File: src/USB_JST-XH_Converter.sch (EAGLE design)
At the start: 47 parts, among them SW1 SS-12D00G3, U1 TCKE805NAWSON10B_TOS-REC, U2 TLP293

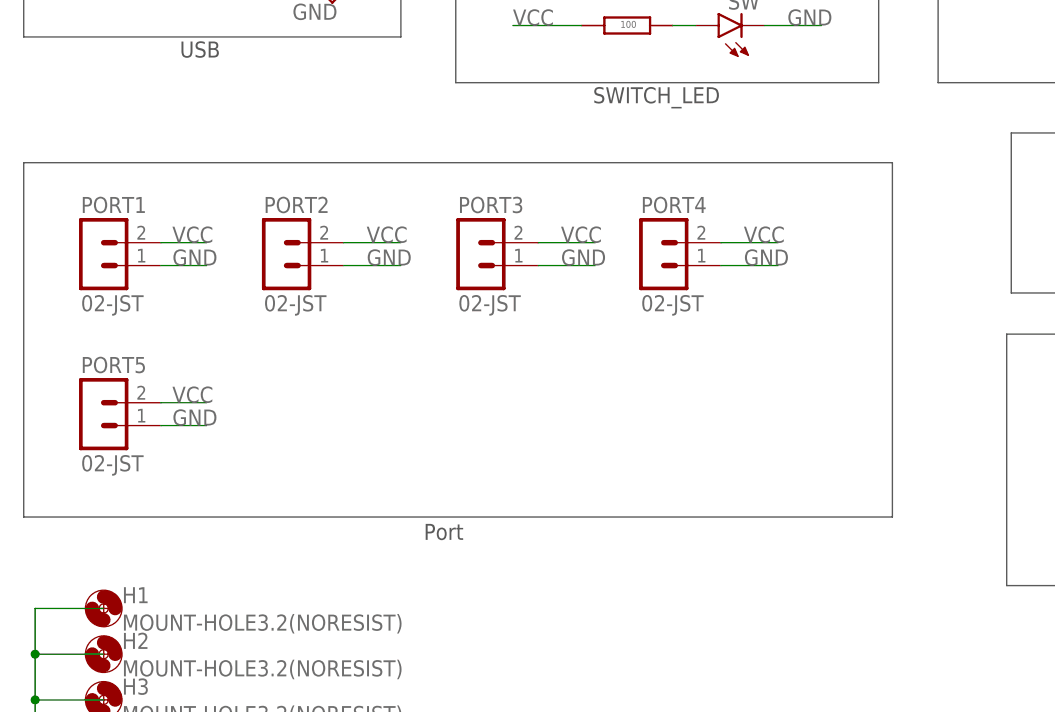
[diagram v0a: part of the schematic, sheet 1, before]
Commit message: 配線完了
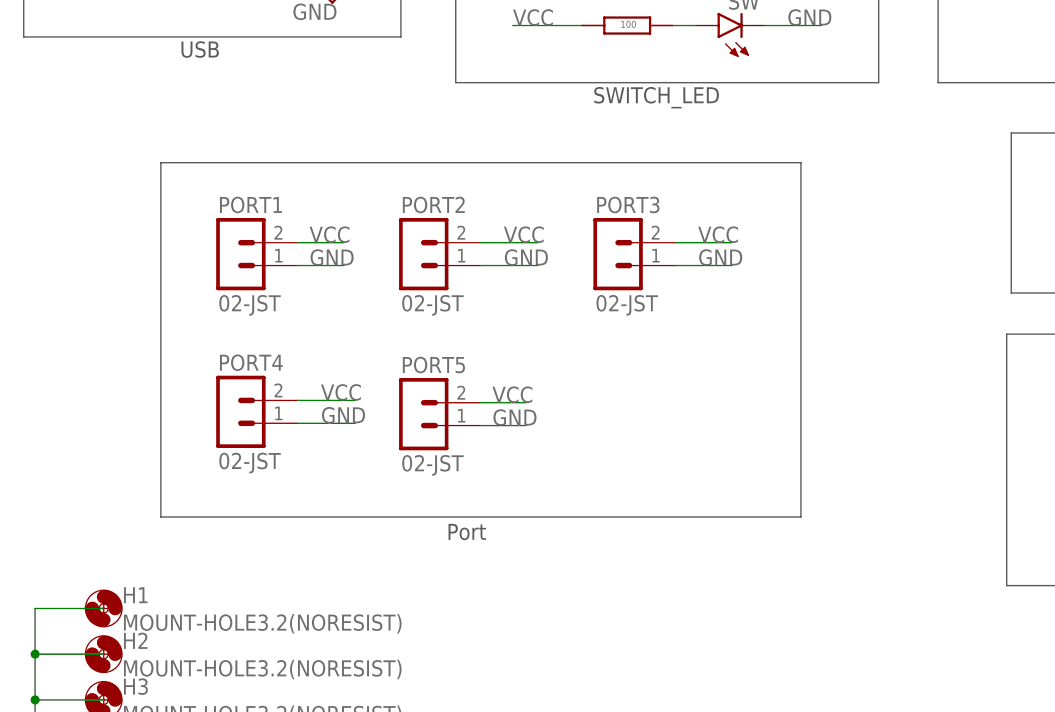
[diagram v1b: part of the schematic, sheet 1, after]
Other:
- moved on the sheet: PORT1, PORT2, PORT3, PORT4, PORT5
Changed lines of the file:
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@@
 <sheet>
 <plain>
-<wire x1="8.89" y1="74.93" x2="8.89" y2="35.56" width="0.1524" layer="97"/>
-<wire x1="8.89" y1="35.56" x2="105.41" y2="35.56" width="0.1524" layer="97"/>
-<wire x1="105.41" y1="35.56" x2="105.41" y2="74.93" width="0.1524" layer="97"/>
-<wire x1="105.41" y1="74.93" x2="8.89" y2="74.93" width="0.1524" layer="97"/>
+<wire x1="24.13" y1="74.93" x2="24.13" y2="35.56" width="0.1524" layer="97"/>
+<wire x1="24.13" y1="35.56" x2="95.25" y2="35.56" width="0.1524" layer="97"/>
+<wire x1="95.25" y1="35.56" x2="95.25" y2="74.93" width="0.1524" layer="97"/>
+<wire x1="95.25" y1="74.93" x2="24.13" y2="74.93" width="0.1524" layer="97"/>
 <wire x1="118.11" y1="55.88" x2="118.11" y2="27.94" width="0.1524" layer="97"/>
 <wire x1="118.11" y1="27.94" x2="170.18" y2="27.94" width="0.1524" layer="97"/>
@@
 <wire x1="170.18" y1="55.88" x2="118.11" y2="55.88" width="0.1524" layer="97"/>
 <text x="139.7" y="25.4" size="1.778" layer="97">Switch</text>
-<text x="53.34" y="33.02" size="1.778" layer="97">Port</text>
+<text x="55.88" y="33.02" size="1.778" layer="97">Port</text>
 <text x="30.734" y="86.614" size="1.778" layer="97" rot="MR0">USB</text>
 <wire x1="56.896" y1="97.79" x2="56.896" y2="83.82" width="0.1524" layer="97"/>
@@
 <attribute name="SHEET" x="154.305" y="5.08" size="2.54" layer="94"/>
 </instance>
-<instance part="PORT1" gate="G$1" x="16.51" y="66.04" smashed="yes">
-<attribute name="VALUE" x="15.24" y="58.42" size="1.778" layer="96"/>
-<attribute name="NAME" x="15.24" y="69.342" size="1.778" layer="95"/>
-</instance>
-<instance part="PORT2" gate="G$1" x="36.83" y="66.04" smashed="yes">
-<attribute name="VALUE" x="35.56" y="58.42" size="1.778" layer="96"/>
-<attribute name="NAME" x="35.56" y="69.342" size="1.778" layer="95"/>
-</instance>
-<instance part="PORT3" gate="G$1" x="58.42" y="66.04" smashed="yes">
-<attribute name="VALUE" x="57.15" y="58.42" size="1.778" layer="96"/>
-<attribute name="NAME" x="57.15" y="69.342" size="1.778" layer="95"/>
-</instance>
-<instance part="PORT4" gate="G$1" x="78.74" y="66.04" smashed="yes">
-<attribute name="VALUE" x="77.47" y="58.42" size="1.778" layer="96"/>
-<attribute name="NAME" x="77.47" y="69.342" size="1.778" layer="95"/>
-</instance>
-<instance part="PORT5" gate="G$1" x="16.51" y="48.26" smashed="yes">
-<attribute name="VALUE" x="15.24" y="40.64" size="1.778" layer="96"/>
-<attribute name="NAME" x="15.24" y="51.562" size="1.778" layer="95"/>
+<instance part="PORT1" gate="G$1" x="31.75" y="66.04" smashed="yes">
+<attribute name="VALUE" x="30.48" y="58.42" size="1.778" layer="96"/>
+<attribute name="NAME" x="30.48" y="69.342" size="1.778" layer="95"/>
+</instance>
+<instance part="PORT2" gate="G$1" x="52.07" y="66.04" smashed="yes">
+<attribute name="VALUE" x="50.8" y="58.42" size="1.778" layer="96"/>
+<attribute name="NAME" x="50.8" y="69.342" size="1.778" layer="95"/>
+</instance>
+<instance part="PORT3" gate="G$1" x="73.66" y="66.04" smashed="yes">
+<attribute name="VALUE" x="72.39" y="58.42" size="1.778" layer="96"/>
+<attribute name="NAME" x="72.39" y="69.342" size="1.778" layer="95"/>
+</instance>
+<instance part="PORT4" gate="G$1" x="31.75" y="48.514" smashed="yes">
+<attribute name="VALUE" x="30.48" y="40.894" size="1.778" layer="96"/>
+<attribute name="NAME" x="30.48" y="51.816" size="1.778" layer="95"/>
+</instance>
+<instance part="PORT5" gate="G$1" x="52.07" y="48.26" smashed="yes">
+<attribute name="VALUE" x="50.8" y="40.64" size="1.778" layer="96"/>
+<attribute name="NAME" x="50.8" y="51.562" size="1.778" layer="95"/>
 </instance>
 <instance part="SW1" gate="G$1" x="143.51" y="43.18" smashed="yes" rot="R270">
@@
 <segment>
 <pinref part="PORT1" gate="G$1" pin="2"/>
-<wire x1="24.13" y1="66.04" x2="29.21" y2="66.04" width="0.1524" layer="91"/>
-<label x="25.4" y="66.04" size="1.778" layer="95"/>
+<wire x1="39.37" y1="66.04" x2="44.45" y2="66.04" width="0.1524" layer="91"/>
+<label x="40.64" y="66.04" size="1.778" layer="95"/>
 </segment>
 <segment>
 <pinref part="PORT2" gate="G$1" pin="2"/>
-<wire x1="44.45" y1="66.04" x2="50.8" y2="66.04" width="0.1524" layer="91"/>
-<label x="46.99" y="66.04" size="1.778" layer="95"/>
+<wire x1="59.69" y1="66.04" x2="66.04" y2="66.04" width="0.1524" layer="91"/>
+<label x="62.23" y="66.04" size="1.778" layer="95"/>
 </segment>
 <segment>
 <pinref part="PORT3" gate="G$1" pin="2"/>
-<wire x1="66.04" y1="66.04" x2="72.39" y2="66.04" width="0.1524" layer="91"/>
-<label x="68.58" y="66.04" size="1.778" layer="95"/>
+<wire x1="81.28" y1="66.04" x2="87.63" y2="66.04" width="0.1524" layer="91"/>
+<label x="83.82" y="66.04" size="1.778" layer="95"/>
 </segment>
 <segment>
 <pinref part="PORT4" gate="G$1" pin="2"/>
-<wire x1="86.36" y1="66.04" x2="92.71" y2="66.04" width="0.1524" layer="91"/>
-<label x="88.9" y="66.04" size="1.778" layer="95"/>
+<wire x1="39.37" y1="48.514" x2="45.72" y2="48.514" width="0.1524" layer="91"/>
+<label x="41.91" y="48.514" size="1.778" layer="95"/>
 </segment>
 <segment>
 <pinref part="PORT5" gate="G$1" pin="2"/>
-<wire x1="24.13" y1="48.26" x2="29.21" y2="48.26" width="0.1524" layer="91"/>
-<label x="25.4" y="48.26" size="1.778" layer="95"/>
+<wire x1="59.69" y1="48.26" x2="64.77" y2="48.26" width="0.1524" layer="91"/>
+<label x="60.96" y="48.26" size="1.778" layer="95"/>
 </segment>
 <segment>
@@
 <segment>
 <pinref part="PORT5" gate="G$1" pin="1"/>
-<wire x1="24.13" y1="45.72" x2="29.21" y2="45.72" width="0.1524" layer="91"/>
-<label x="25.4" y="45.72" size="1.778" layer="95"/>
+<wire x1="59.69" y1="45.72" x2="64.77" y2="45.72" width="0.1524" layer="91"/>
+<label x="60.96" y="45.72" size="1.778" layer="95"/>
 </segment>
 <segment>
 <pinref part="PORT1" gate="G$1" pin="1"/>
-<wire x1="24.13" y1="63.5" x2="29.21" y2="63.5" width="0.1524" layer="91"/>
-<label x="25.4" y="63.5" size="1.778" layer="95"/>
+<wire x1="39.37" y1="63.5" x2="44.45" y2="63.5" width="0.1524" layer="91"/>
+<label x="40.64" y="63.5" size="1.778" layer="95"/>
 </segment>
 <segment>
 <pinref part="PORT2" gate="G$1" pin="1"/>
-<wire x1="44.45" y1="63.5" x2="50.8" y2="63.5" width="0.1524" layer="91"/>
-<label x="46.99" y="63.5" size="1.778" layer="95"/>
+<wire x1="59.69" y1="63.5" x2="66.04" y2="63.5" width="0.1524" layer="91"/>
+<label x="62.23" y="63.5" size="1.778" layer="95"/>
 </segment>
 <segment>
 <pinref part="PORT3" gate="G$1" pin="1"/>
-<wire x1="66.04" y1="63.5" x2="72.39" y2="63.5" width="0.1524" layer="91"/>
-<label x="68.58" y="63.5" size="1.778" layer="95"/>
+<wire x1="81.28" y1="63.5" x2="87.63" y2="63.5" width="0.1524" layer="91"/>
+<label x="83.82" y="63.5" size="1.778" layer="95"/>
 </segment>
 <segment>
 <pinref part="PORT4" gate="G$1" pin="1"/>
-<wire x1="86.36" y1="63.5" x2="92.71" y2="63.5" width="0.1524" layer="91"/>
-<label x="88.9" y="63.5" size="1.778" layer="95"/>
-</segment>
-<segment>
+<wire x1="39.37" y1="45.974" x2="45.72" y2="45.974" width="0.1524" layer="91"/>
+<label x="41.91" y="45.974" size="1.778" layer="95"/>
+</segment>
+<segment>
